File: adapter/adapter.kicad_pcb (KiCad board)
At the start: 2 copper layers, 61.4 x 50.9 mm, 42 parts, among them J1 Serial, J10 Ribbon, J11 Ribbon, J12 Ribbon, J2 Serial, J3 battery charge, J4 RGB, J5 RGB, J6 battery charge, J7 trackball, J8 trackball, J9 Ribbon, SW1 SW_SPST, SW2 SW_SPST, SW3 SW_SPDT, SW4 SW_SPDT, U1 eliteC, U2 eliteC

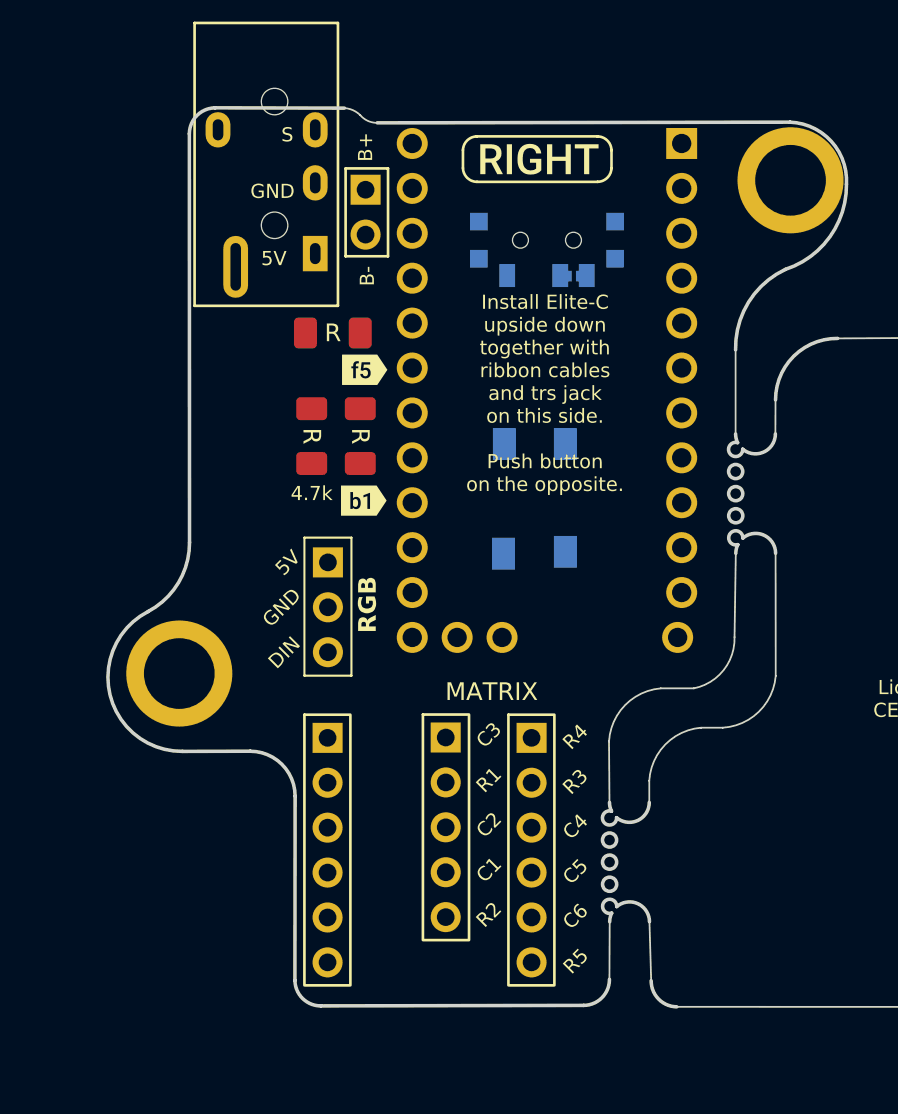
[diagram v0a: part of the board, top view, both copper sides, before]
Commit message: pcb(edge-cuts): symmetry!
Signed-off-by: Anant Thazhemadam <anant.thazhemadam@gmail.com>
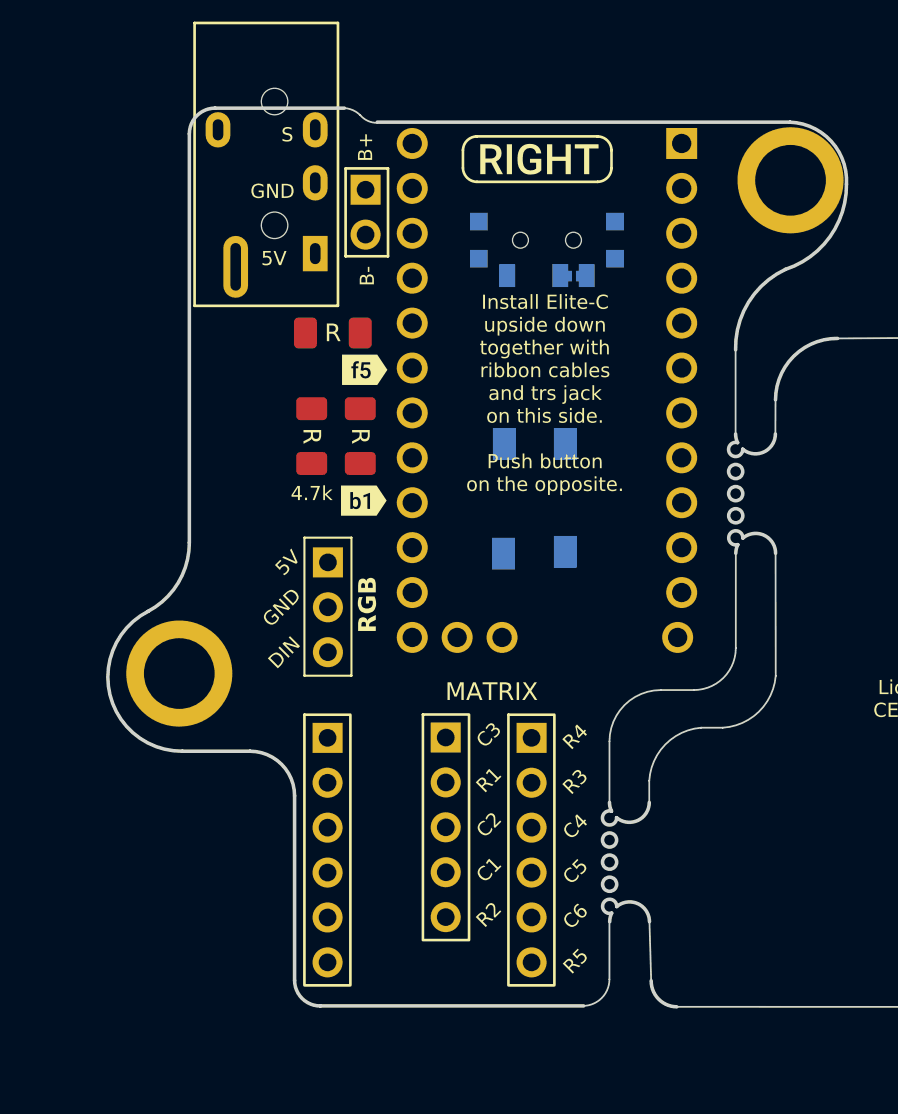
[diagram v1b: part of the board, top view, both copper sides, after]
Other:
- board size 61.4 x 50.9 mm -> 61.4 x 50.8 mm
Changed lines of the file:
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@@
 	)
 	(gr_arc
-		(start 113.341486 91.773749)
-		(mid 112.713926 94.049213)
-		(end 111.001486 95.673749)
+		(start 113.331485 91.773751)
+		(mid 112.705363 94.044066)
+		(end 110.996809 95.664932)
 		(stroke
 			(width 0.2)
@@
 	(gr_line
 		(start 137.096291 106.475003)
-		(end 137.07 103.02)
+		(end 137.096291 103.0199)
+		(locked yes)
 		(stroke
 			(width 0.1)
@@
 	)
 	(gr_line
-		(start 120.775358 117.982362)
-		(end 135.631351 117.953354)
+		(start 120.736124 117.982362)
+		(end 135.631379 117.982362)
 		(stroke
 			(width 0.2)
@@
 	)
 	(gr_line
-		(start 141.87 100.02)
-		(end 139.998866 100.02)
+		(start 141.870036 100.116191)
+		(end 139.998902 100.116191)
+		(locked yes)
 		(stroke
 			(width 0.1)
@@
 		(start 144.230005 85.631645)
 		(end 144.230005 80.872466)
-		(stroke
-			(width 0.1)
-			(type solid)
-		)
-		(layer "Edge.Cuts")
-	)
-	(gr_line
-		(start 112.943471 103.585074)
-		(end 116.773949 103.576051)
-		(stroke
-			(width 0.2)
-			(type solid)
+		(locked yes)
+		(stroke
+			(width 0.1)
+			(type solid)
+		)
+		(layer "Edge.Cuts")
+	)
+	(gr_line
+		(start 112.938794 103.576257)
+		(end 116.769283 103.576257)
+		(locked yes)
+		(stroke
+			(width 0.2)
+			(type solid)
+		)
+		(layer "Edge.Cuts")
+	)
+	(gr_arc
+		(start 120.736124 117.985765)
+		(mid 119.709142 117.560375)
+		(end 119.283752 116.533393)
+		(stroke
+			(width 0.2)
+			(type default)
 		)
 		(layer "Edge.Cuts")
@@
 	)
 	(gr_arc
-		(start 144.17 97.12)
-		(mid 143.551367 98.991429)
-		(end 141.87 100.02)
-		(stroke
-			(width 0.1)
-			(type solid)
+		(start 137.09335 116.477233)
+		(mid 136.652508 117.541521)
+		(end 135.58822 117.982363)
+		(locked yes)
+		(stroke
+			(width 0.1)
+			(type default)
 		)
 		(layer "Edge.Cuts")
@@
 	)
 	(gr_line
-		(start 137.108072 113.224991)
-		(end 137.09335 116.477233)
+		(start 137.09335 113.224991)
+		(end 137.09335 116.477266)
+		(locked yes)
 		(stroke
 			(width 0.1)
@@
 	)
 	(gr_line
-		(start 144.17 97.12)
+		(start 144.241822 97.744405)
 		(end 144.241786 92.381633)
+		(locked yes)
 		(stroke
 			(width 0.1)
@@
 	)
 	(gr_arc
+		(start 116.769283 103.576258)
+		(mid 118.549131 104.317198)
+		(end 119.283752 106.099664)
+		(locked yes)
+		(stroke
+			(width 0.2)
+			(type default)
+		)
+		(layer "Edge.Cuts")
+	)
+	(gr_arc
 		(start 137.210084 106.966079)
 		(mid 137.125328 106.726997)
@@
 		(layer "Edge.Cuts")
 	)
+	(gr_arc
+		(start 137.096291 103.0199)
+		(mid 137.94638 100.967056)
+		(end 139.998902 100.116191)
+		(locked yes)
+		(stroke
+			(width 0.1)
+			(type default)
+		)
+		(layer "Edge.Cuts")
+	)
 	(gr_line
 		(start 147.305648 67.994096)
-		(end 123.961303 68.03306)
+		(end 123.96127 67.994096)
+		(locked yes)
 		(stroke
 			(width 0.2)
@@
 	(gr_line
 		(start 122.1 67.2)
-		(end 114.781486 67.183749)
+		(end 114.785236 67.199999)
+		(locked yes)
 		(stroke
 			(width 0.2)
@@
 	)
 	(gr_arc
-		(start 112.943471 103.585074)
-		(mid 108.84637 100.396774)
-		(end 111.001486 95.673749)
+		(start 112.938794 103.576257)
+		(mid 108.841727 100.387977)
+		(end 110.996809 95.664932)
 		(stroke
 			(width 0.2)
@@
 	(gr_arc
 		(start 113.331486 68.653749)
-		(mid 113.754912 67.621278)
-		(end 114.781486 67.183749)
-		(stroke
-			(width 0.2)
-			(type solid)
+		(mid 113.75728 67.625793)
+		(end 114.785236 67.199999)
+		(locked yes)
+		(stroke
+			(width 0.2)
+			(type default)
 		)
 		(layer "Edge.Cuts")
@@
 	)
 	(gr_line
-		(start 119.302824 116.533393)
-		(end 119.313949 106.116051)
-		(stroke
-			(width 0.2)
-			(type solid)
-		)
-		(layer "Edge.Cuts")
-	)
-	(gr_arc
-		(start 137.09335 116.477233)
-		(mid 136.67 117.52)
-		(end 135.631351 117.953354)
-		(stroke
-			(width 0.2)
-			(type solid)
-		)
-		(layer "Edge.Cuts")
-	)
-	(gr_arc
-		(start 120.775358 117.982362)
-		(mid 119.738483 117.563374)
-		(end 119.302824 116.533393)
+		(start 119.283752 116.533393)
+		(end 119.283752 106.099664)
+		(locked yes)
 		(stroke
 			(width 0.2)
@@
 		(stroke
 			(width 0.1)
-			(type solid)
-		)
-		(layer "Edge.Cuts")
-	)
-	(gr_arc
-		(start 116.773949 103.576051)
-		(mid 118.57 104.32)
-		(end 119.313949 106.116051)
-		(stroke
-			(width 0.2)
 			(type solid)
 		)
@@
 	)
 	(gr_arc
+		(start 144.241822 97.744405)
+		(mid 143.547142 99.421511)
+		(end 141.870036 100.116191)
+		(locked yes)
+		(stroke
+			(width 0.1)
+			(type default)
+		)
+		(layer "Edge.Cuts")
+	)
+	(gr_arc
 		(start 137.108072 113.224991)
 		(mid 137.136229 112.972898)
@@
 	)
 	(gr_arc
-		(start 137.07 103.02)
-		(mid 137.974475 100.973319)
-		(end 139.998866 100.02)
-		(stroke
-			(width 0.1)
-			(type solid)
-		)
-		(layer "Edge.Cuts")
-	)
-	(gr_arc
 		(start 140.903204 118.03399)
 		(mid 139.873005 117.596021)
@@
 	(gr_line
 		(start 113.331486 68.653749)
-		(end 113.341486 91.773749)
-		(stroke
-			(width 0.2)
+		(end 113.331486 91.773751)
+		(locked yes)
+		(stroke
+			(width 0.2)
